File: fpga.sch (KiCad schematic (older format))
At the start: 57 parts, among them P1 JTAG, SW2 BTN0, U10 S25FL216K, U12 TLV70012, U13 TLV70025, U14 TLV70012, U2 EP4CE15E22

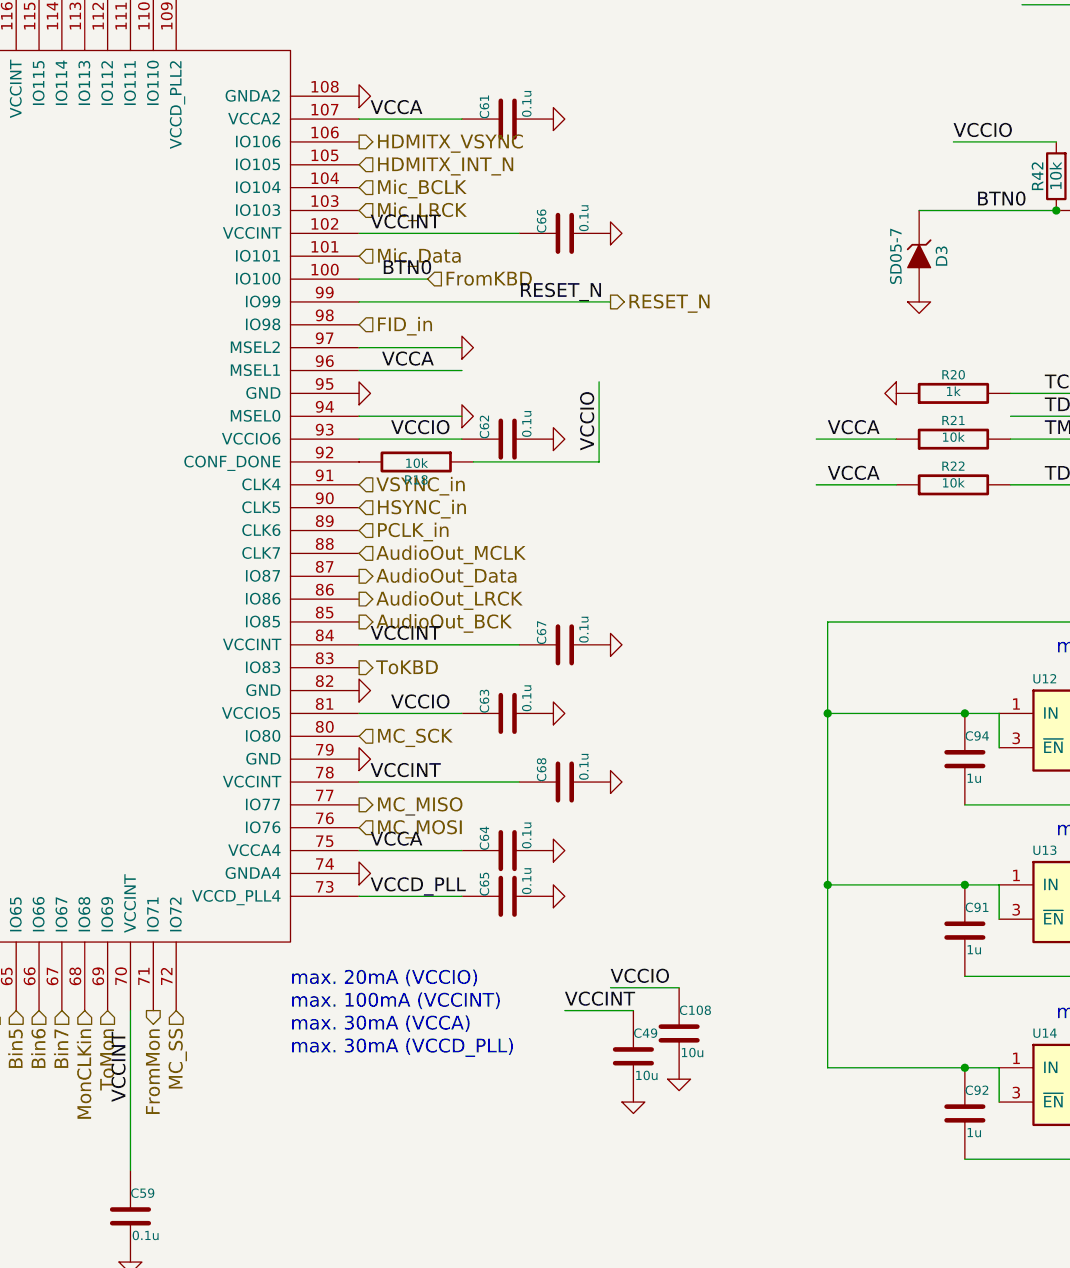
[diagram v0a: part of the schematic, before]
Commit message: update PCB
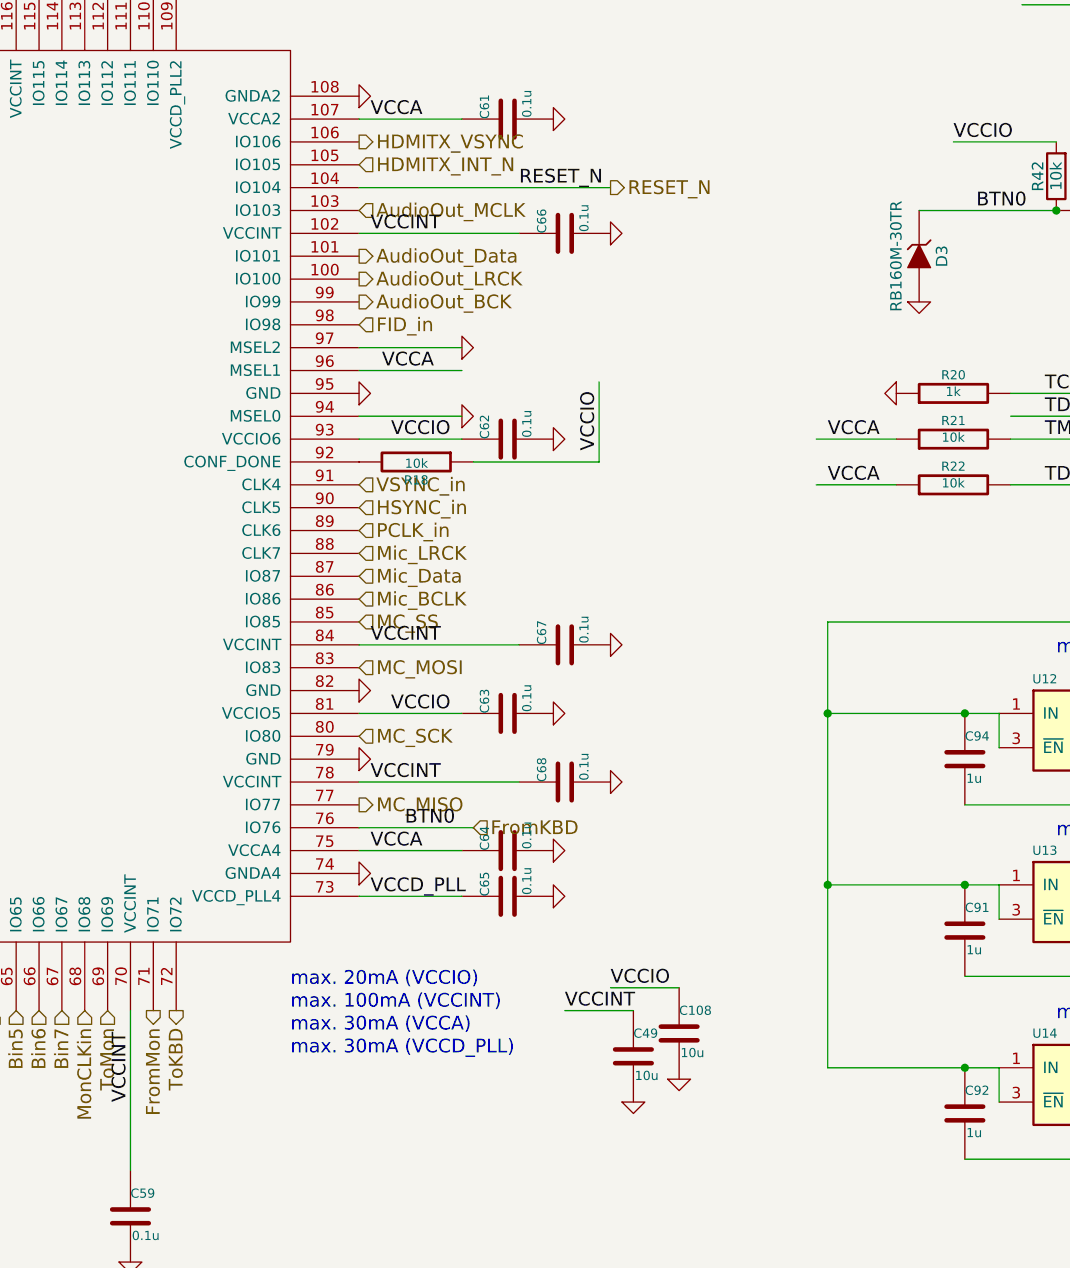
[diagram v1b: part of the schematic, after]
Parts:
- D3: value SD05-7 -> RB160M-30TR; footprint Diode_SMD:D_SOD-323_HandSoldering -> custom_components:D_SOD-123_HandSoldering
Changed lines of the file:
@@
 Text HLabel 6800 3350 2    60   Input ~ 0
 FID_in
-Text HLabel 7900 3250 2    60   Output ~ 0
+Text HLabel 7900 2750 2    60   Output ~ 0
 RESET_N
 Text HLabel 6800 2650 2    60   Input ~ 0
@@
 	10050 5450 10050 5400
 Wire Wire Line
-	8850 5050 9450 5050
-Wire Wire Line
 	9600 5050 9600 5200
 Connection ~ 9450 5050
@@
 	8850 4650 10850 4650
 Wire Wire Line
-	6800 3250 7900 3250
+	6800 2750 7900 2750
 Connection ~ 10350 1100
 Wire Wire Line
@@
 Text Label 9400 2550 0    60   ~ 0
 VCCIO
-Text Label 6900 3150 0    60   ~ 0
+Text Label 7000 5550 0    60   ~ 0
 BTN0
 Wire Wire Line
@@
 Text Notes 6500 6550 0    60   ~ 0
 max. 30mA (VCCD_PLL)
-Text Label 7500 3250 0    60   ~ 0
+Text Label 7500 2750 0    60   ~ 0
 RESET_N
 $Comp
@@
 VCCIO
 $Comp
-L ossc_board-rescue:ZENER D3
-U 1 1 58C560B1
-P 9250 3050
-F 0 "D3" H 9250 3150 50  0000 C CNN
-F 1 "SD05-7" H 9250 2950 50  0000 C CNN
-F 2 "Diode_SMD:D_SOD-323_HandSoldering" H 9250 3050 60  0001 C CNN
-F 3 "" H 9250 3050 60  0000 C CNN
-	1    9250 3050
-	0    1    1    0
-$EndComp
-$Comp
 L ossc_board-rescue:GND-RESCUE-ossc_board #PWR078
 U 1 1 58C561E6
@@
 Text HLabel 5900 6350 3    60   Output ~ 0
 FromMon
-Text HLabel 6000 6350 3    60   Input ~ 0
+Text HLabel 6800 4650 2    60   Input ~ 0
 MC_SS
-Text HLabel 6800 5550 2    60   Input ~ 0
+Text HLabel 6800 4850 2    60   Input ~ 0
 MC_MOSI
 Text HLabel 6800 5450 2    60   Output ~ 0
@@
 Text HLabel 6800 5150 2    60   Input ~ 0
 MC_SCK
+Text HLabel 6800 2850 2    60   Input ~ 0
+AudioOut_MCLK
+Text HLabel 6800 3250 2    60   Output ~ 0
+AudioOut_BCK
+Text HLabel 6800 3150 2    60   Output ~ 0
+AudioOut_LRCK
+Text HLabel 6800 3050 2    60   Output ~ 0
+AudioOut_Data
+Text HLabel 6800 4550 2    60   Input ~ 0
+Mic_BCLK
 Text HLabel 6800 4350 2    60   Input ~ 0
-AudioOut_MCLK
-Text HLabel 6800 4650 2    60   Output ~ 0
-AudioOut_BCK
-Text HLabel 6800 4550 2    60   Output ~ 0
-AudioOut_LRCK
-Text HLabel 6800 4450 2    60   Output ~ 0
-AudioOut_Data
-Text HLabel 6800 2750 2    60   Input ~ 0
-Mic_BCLK
-Text HLabel 6800 2850 2    60   Input ~ 0
 Mic_LRCK
-Text HLabel 6800 3050 2    60   Input ~ 0
+Text HLabel 6800 4450 2    60   Input ~ 0
 Mic_Data
 Text HLabel 1300 4550 0    60   Output ~ 0
 SPDIF_OUT
-Wire Wire Line
-	7100 3150 6800 3150
-Text HLabel 7100 3150 2    60   Input ~ 0
+Text HLabel 7300 5550 2    60   Input ~ 0
 FromKBD
-Text HLabel 6800 4850 2    60   Output ~ 0
+Text HLabel 6000 6350 3    60   Output ~ 0
 ToKBD
+Wire Wire Line
+	6800 5550 7300 5550
+$Comp
+L ossc_board-rescue:ZENER D3
+U 1 1 58C560B1
+P 9250 3050
+F 0 "D3" H 9250 3150 50  0000 C CNN
+F 1 "RB160M-30TR" H 9250 2950 50  0000 C CNN
+F 2 "custom_components:D_SOD-123_HandSoldering" H 9250 3050 60  0001 C CNN
+F 3 "" H 9250 3050 60  0000 C CNN
+	1    9250 3050
+	0    1    1    0
+$EndComp
+Wire Wire Line
+	8850 5050 9450 5050
 $EndSCHEMATC
